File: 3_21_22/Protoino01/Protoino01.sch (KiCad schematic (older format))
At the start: 54 parts, among them J1 USB_C_Receptacle_USB2.0, J2 ICSP, SW1 RESET, SW2 SW1, SW3 SW2, U1 ATmega328P-AU, U2 CH340C, U3 74HC14, Y1 16MHz

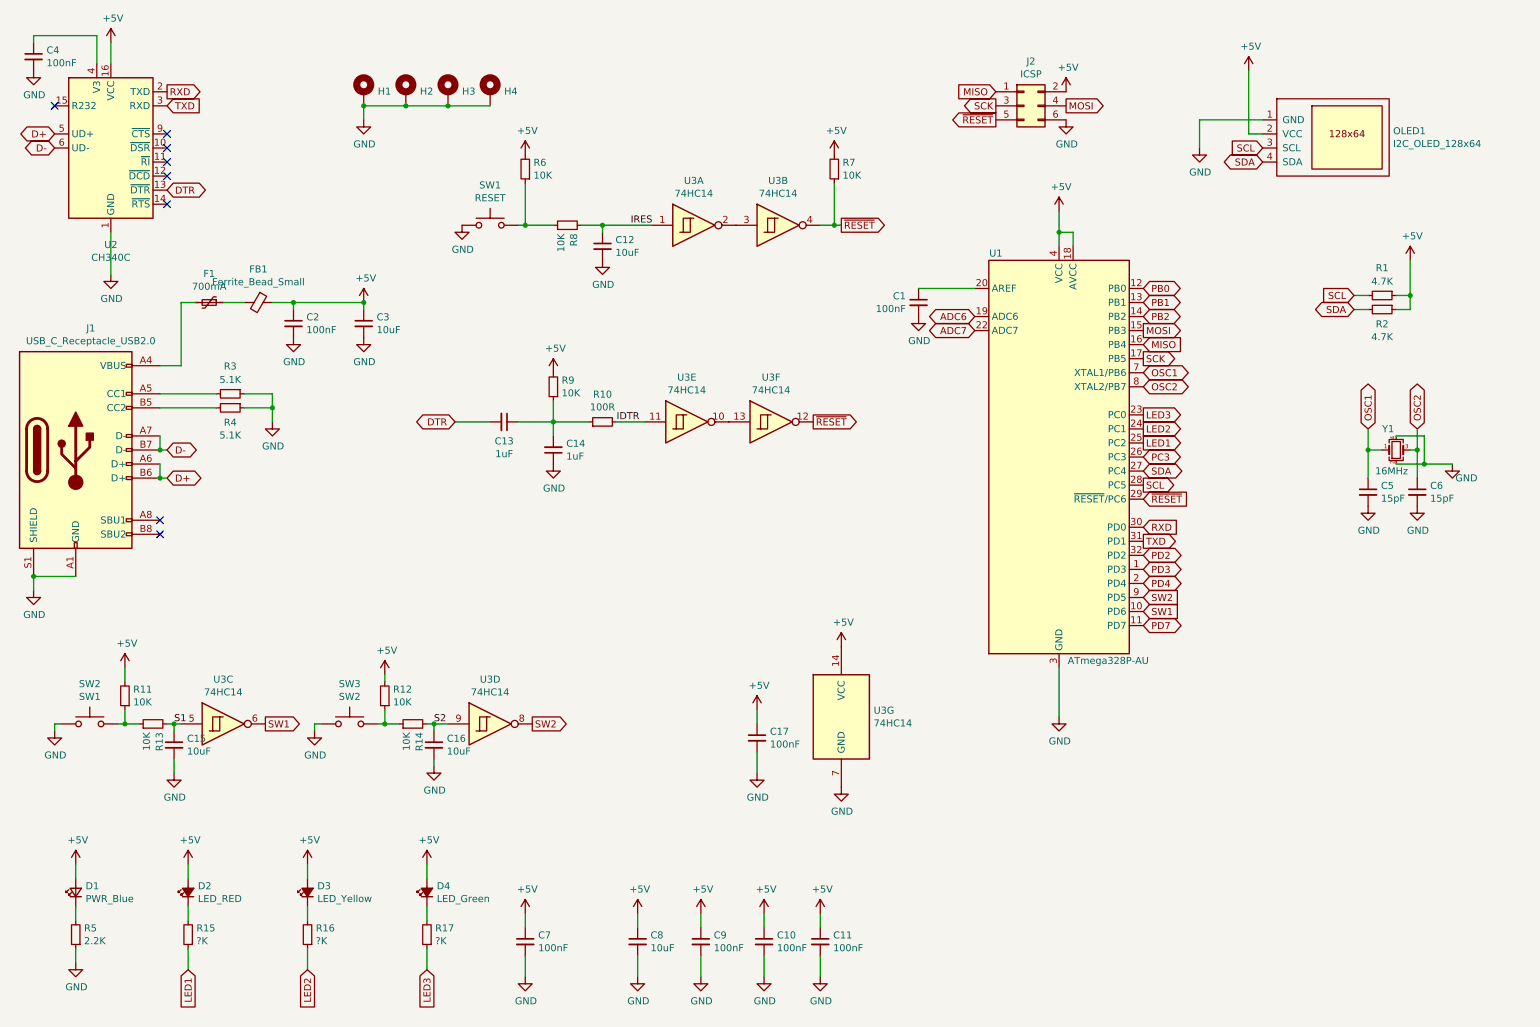
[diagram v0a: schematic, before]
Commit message: Finished Protoino
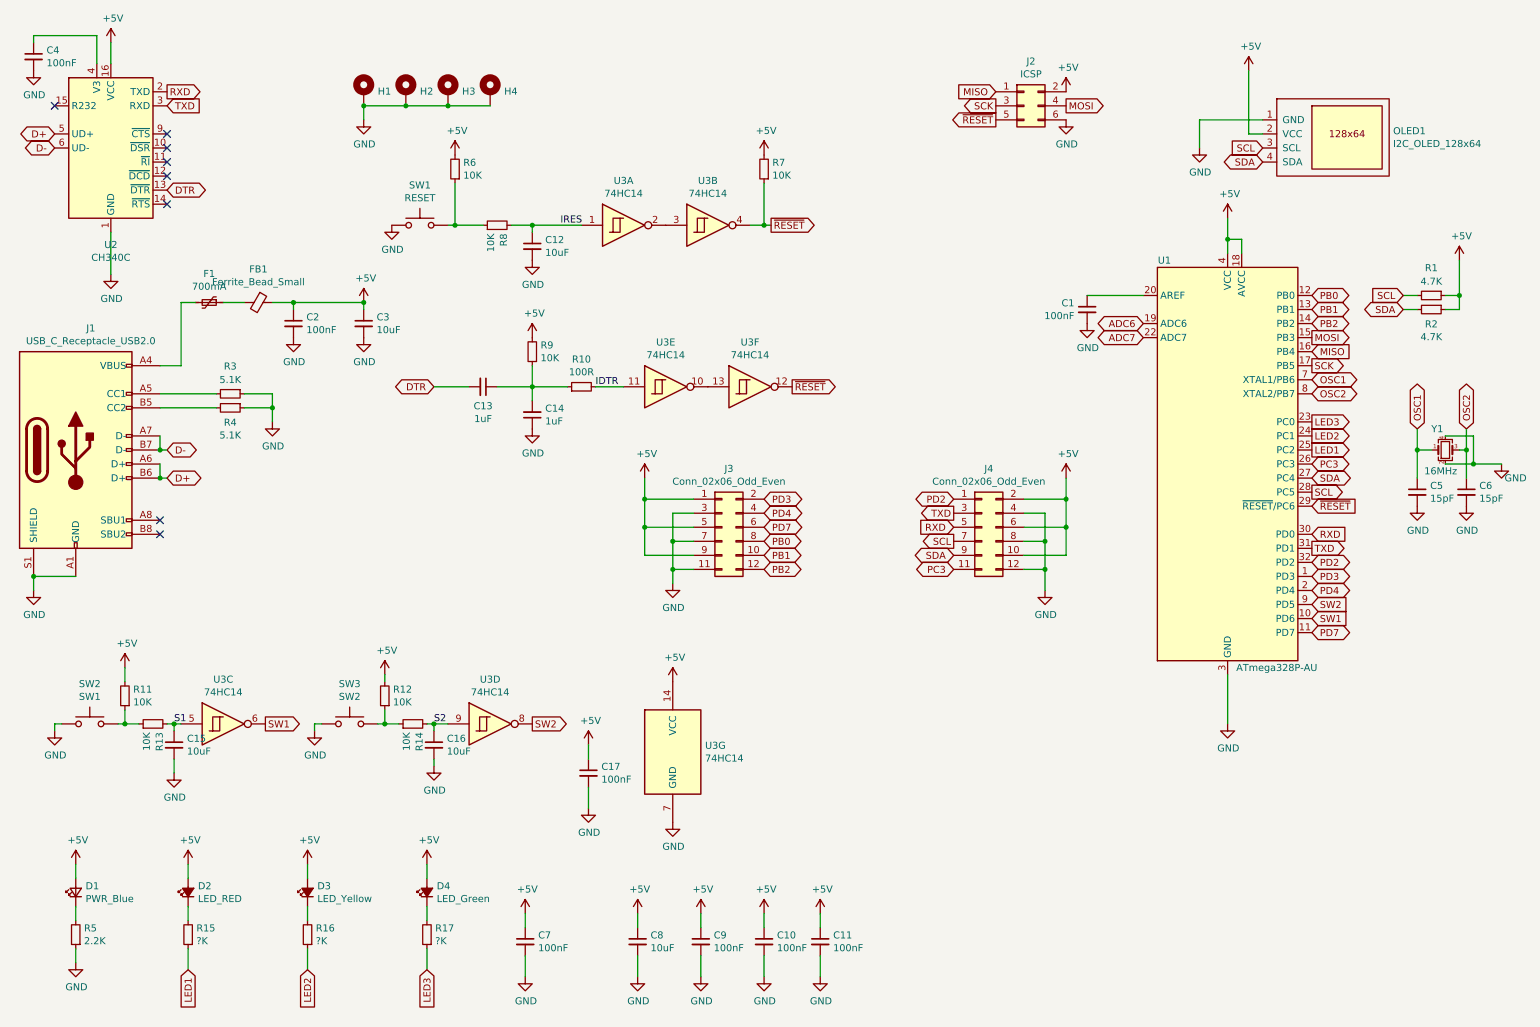
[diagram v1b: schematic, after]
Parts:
- added J3, J4: Conn_02x06_Odd_Even, Connector_PinHeader_2.54mm:PinHeader_2x06_P2.54mm_Vertical, symbol Connector_Generic:Conn_02x06_Odd_Even
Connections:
- net +5V: now also J3.1 (Pin_1), J3.5 (Pin_5), J3.9 (Pin_9), J4.10 (Pin_10), J4.2 (Pin_2), J4.6 (Pin_6)
- net GND: now also J3.11 (Pin_11), J3.3 (Pin_3), J3.7 (Pin_7), J4.12 (Pin_12), J4.4 (Pin_4), J4.8 (Pin_8)
- net PB0: now also J3.8 (Pin_8)
- net PB1: now also J3.10 (Pin_10)
- net PB2: now also J3.12 (Pin_12)
- net PC3: now also J4.11 (Pin_11)
- net PD2: now also J4.1 (Pin_1)
- net PD3: now also J3.2 (Pin_2)
- net PD4: now also J3.4 (Pin_4)
- net PD7: now also J3.6 (Pin_6)
- net RXD: now also J4.5 (Pin_5)
- net SCL: now also J4.7 (Pin_7)
- net SDA: now also J4.9 (Pin_9)
- net TXD: now also J4.3 (Pin_3)
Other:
- moved on the sheet: C1, C12, C13, C14, C17, C5, C6, R1, R10, R2, R6, R7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
